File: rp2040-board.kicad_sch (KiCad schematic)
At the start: 88 parts, among them J1 24V IN, J10 E0-RUNOUT, J11 FAN1, J12 FAN2, J13 FAN3, J14 HB, J15 E0, J16 TH-E0, J2 USB4105-GF-A, J3 PGA2040, J4 3_GPIO, J5 PROBE, J6 X-ENDSTOP, J7 TH-HB, J8 Y-ENDSTOP, J9 Z-ENDSTOP, Q1 AO3400C, Q2 AO3400C, Q3 AO3400C, U1 AMS1117-3.3, U2 TPS5450DDAR, U3 74HCT365D,653, U4 FDS8896, U5 FDS8896

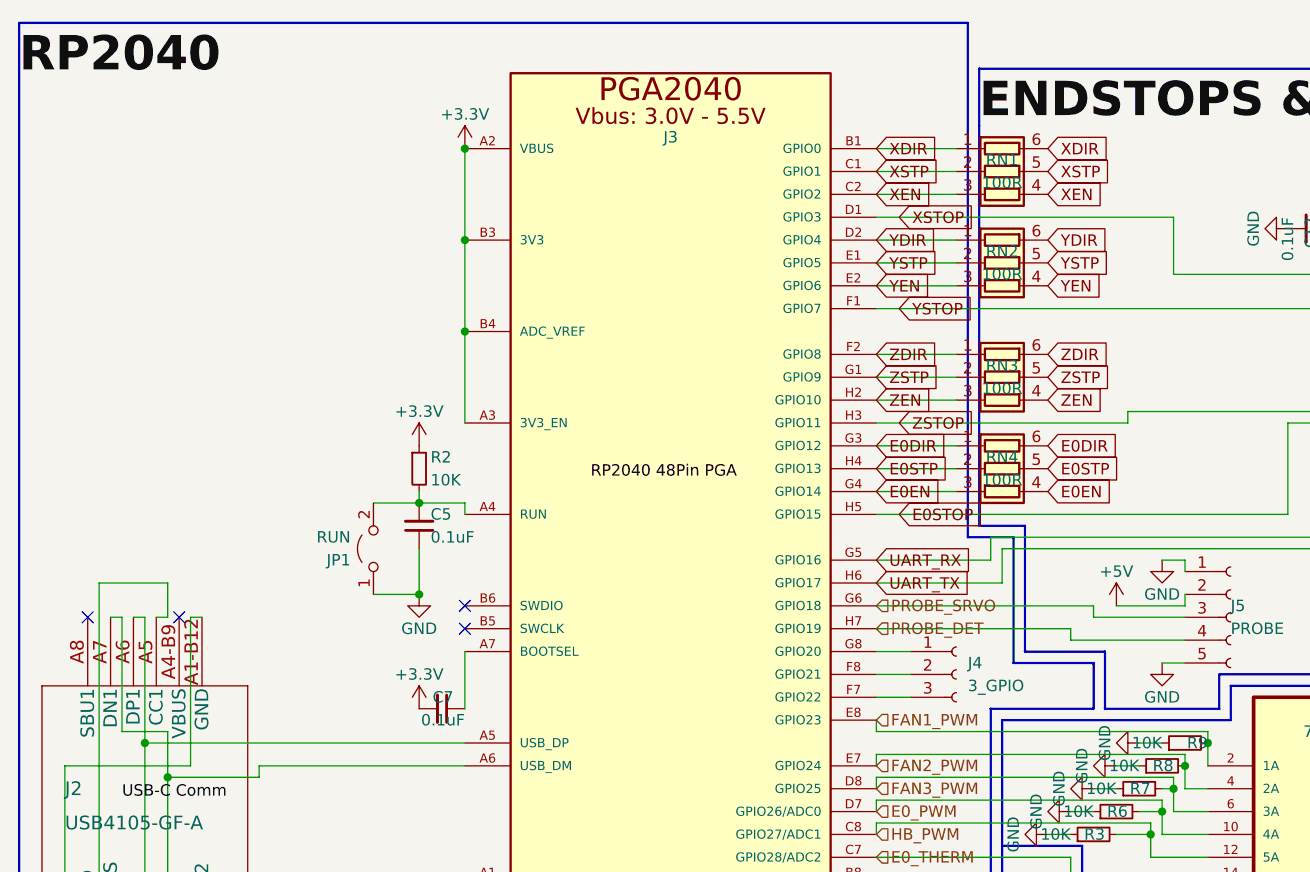
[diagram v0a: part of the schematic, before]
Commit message: finished, for now, finally
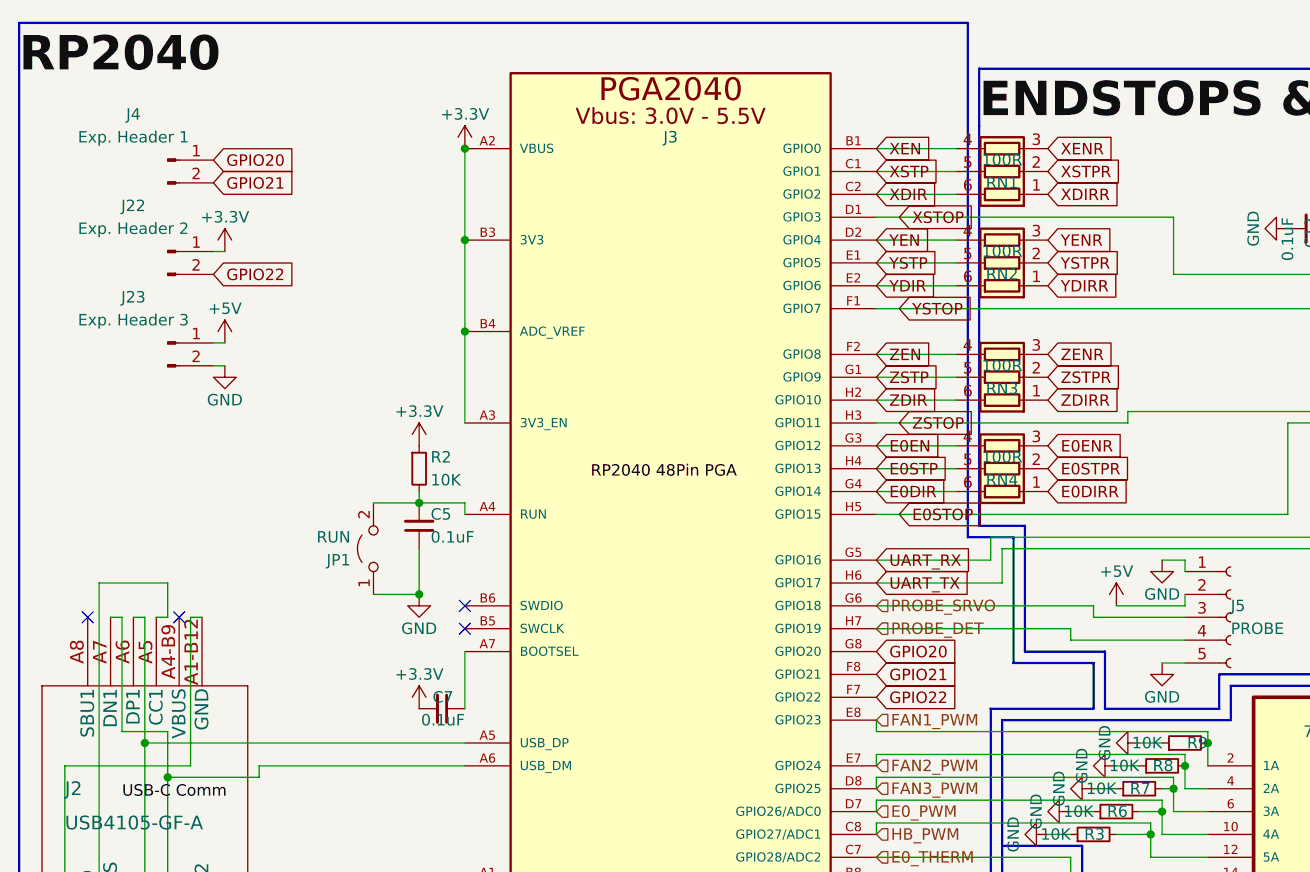
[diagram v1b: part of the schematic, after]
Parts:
- removed J4: 3_GPIO, Connector_PinSocket_2.54mm:PinSocket_1x03_P2.54mm_Vertical, symbol Connector:Conn_01x03_Female
- added J22: Exp. Header 2, Connector_PinHeader_2.54mm:PinHeader_1x02_P2.54mm_Vertical, symbol Connector:Conn_01x02_Male
- added J23: Exp. Header 3, Connector_PinHeader_2.54mm:PinHeader_1x02_P2.54mm_Vertical, symbol Connector:Conn_01x02_Male
- added J4: Exp. Header 1, symbol Connector:Conn_01x02_Male
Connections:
- net +3.3V: now also J22.1 (Pin_1)
- net +5V: now also J23.1 (Pin_1)
- net E0DIR: now also J3.G4 (GPIO14); no longer J3.G3 (GPIO12), RN4.1 (R1.1)
- net E0EN: now also J3.G3 (GPIO12); no longer J3.G4 (GPIO14), RN4.3 (R3.1)
- net E0STP: no longer RN4.2 (R2.1)
- net GND: now also J23.2 (Pin_2)
- net XDIR: now also J3.C2 (GPIO2); no longer J3.B1 (GPIO0), RN1.1 (R1.1)
- net XEN: now also J3.B1 (GPIO0); no longer J3.C2 (GPIO2), RN1.3 (R3.1)
- net XSTP: no longer RN1.2 (R2.1)
- net YDIR: now also J3.E2 (GPIO6); no longer J3.D2 (GPIO4), RN2.1 (R1.1)
- net YEN: now also J3.D2 (GPIO4); no longer J3.E2 (GPIO6), RN2.3 (R3.1)
- net YSTP: no longer RN2.2 (R2.1)
- net ZDIR: now also J3.H2 (GPIO10); no longer J3.F2 (GPIO8), RN3.1 (R1.1)
- net ZEN: now also J3.F2 (GPIO8); no longer J3.H2 (GPIO10), RN3.3 (R3.1)
- net ZSTP: no longer RN3.2 (R2.1)
- net GPIO22: now reaches J3.F7 (GPIO22)
- net GPIO22: now also J22.2 (Pin_2)
- net GPIO21: now reaches J3.F8 (GPIO21)
- net GPIO21: now also J4.2 (Pin_2)
- net GPIO20: now reaches J3.G8 (GPIO20)
- net GPIO20: now also J4.1 (Pin_1)
- new net E0DIRR: RN4.1 (R1.1)
- new net E0ENR: RN4.3 (R3.1)
- new net E0STPR: RN4.2 (R2.1)
- new net XDIRR: RN1.1 (R1.1)
- new net XENR: RN1.3 (R3.1)
- new net XSTPR: RN1.2 (R2.1)
- new net YDIRR: RN2.1 (R1.1)
- new net YENR: RN2.3 (R3.1)
- new net YSTPR: RN2.2 (R2.1)
- new net ZDIRR: RN3.1 (R1.1)
- new net ZENR: RN3.3 (R3.1)
- new net ZSTPR: RN3.2 (R2.1)
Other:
- moved on the sheet: RN1, RN2, RN3, RN4
